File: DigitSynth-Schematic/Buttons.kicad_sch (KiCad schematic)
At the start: 16 parts

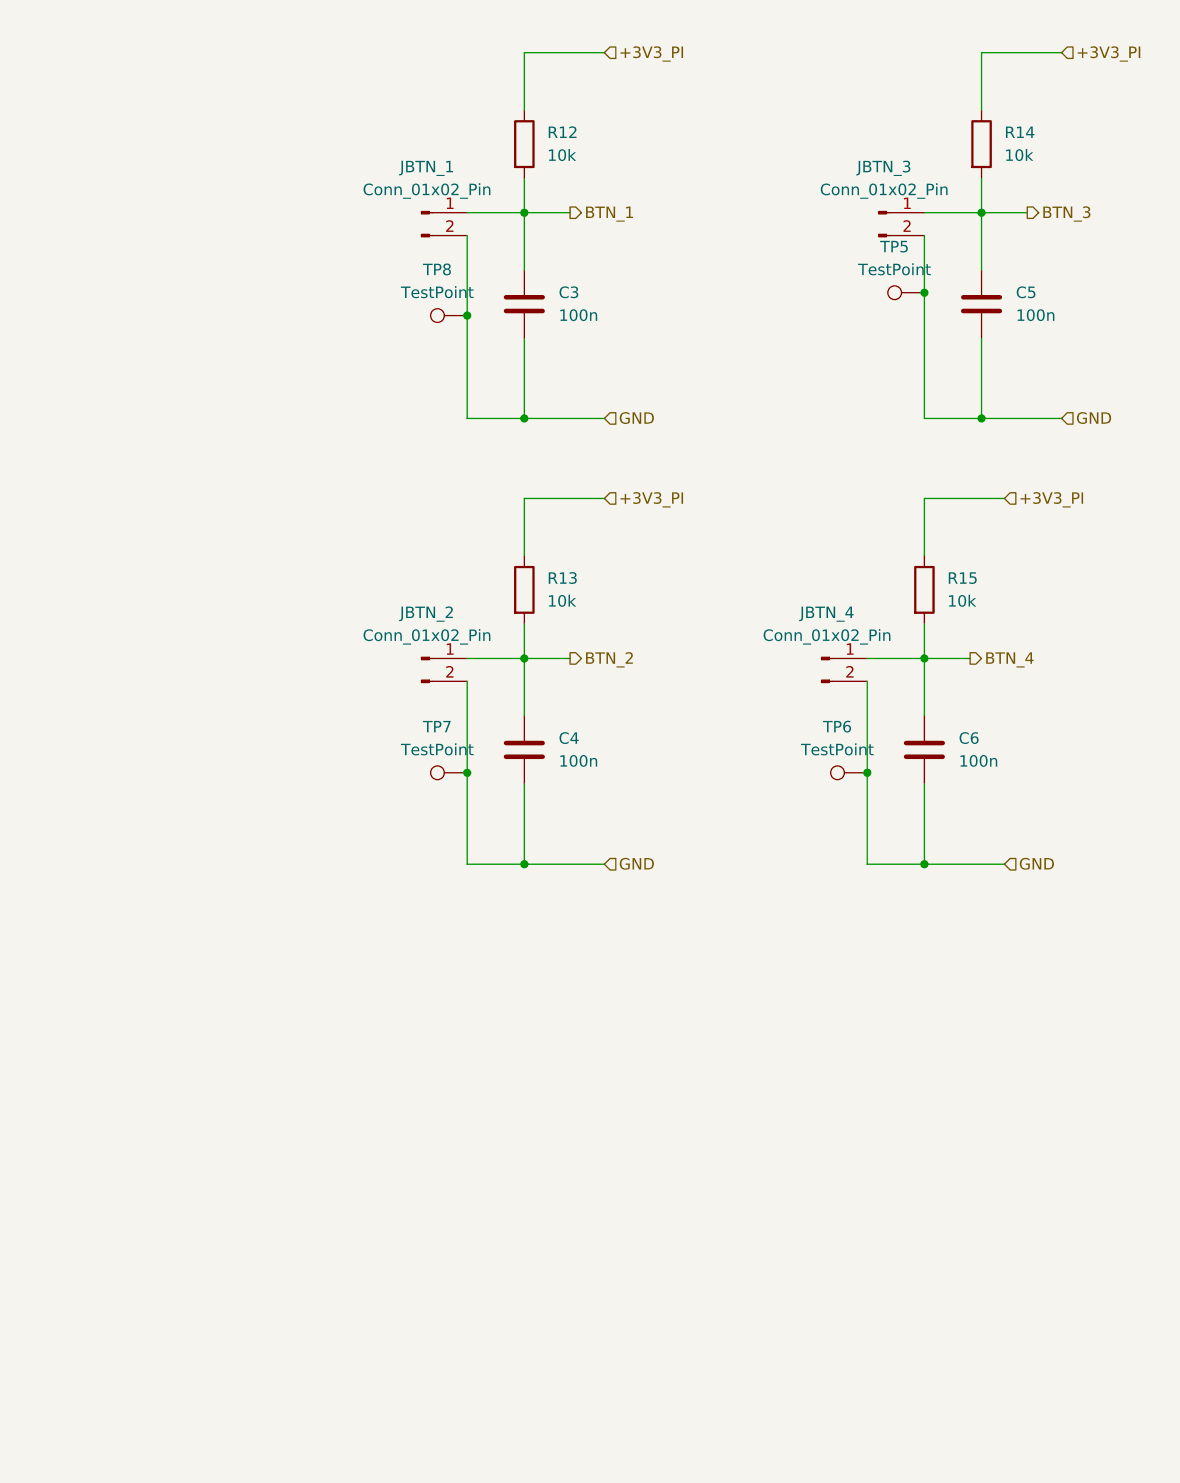
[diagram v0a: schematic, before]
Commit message: KiCad PCB fully routed
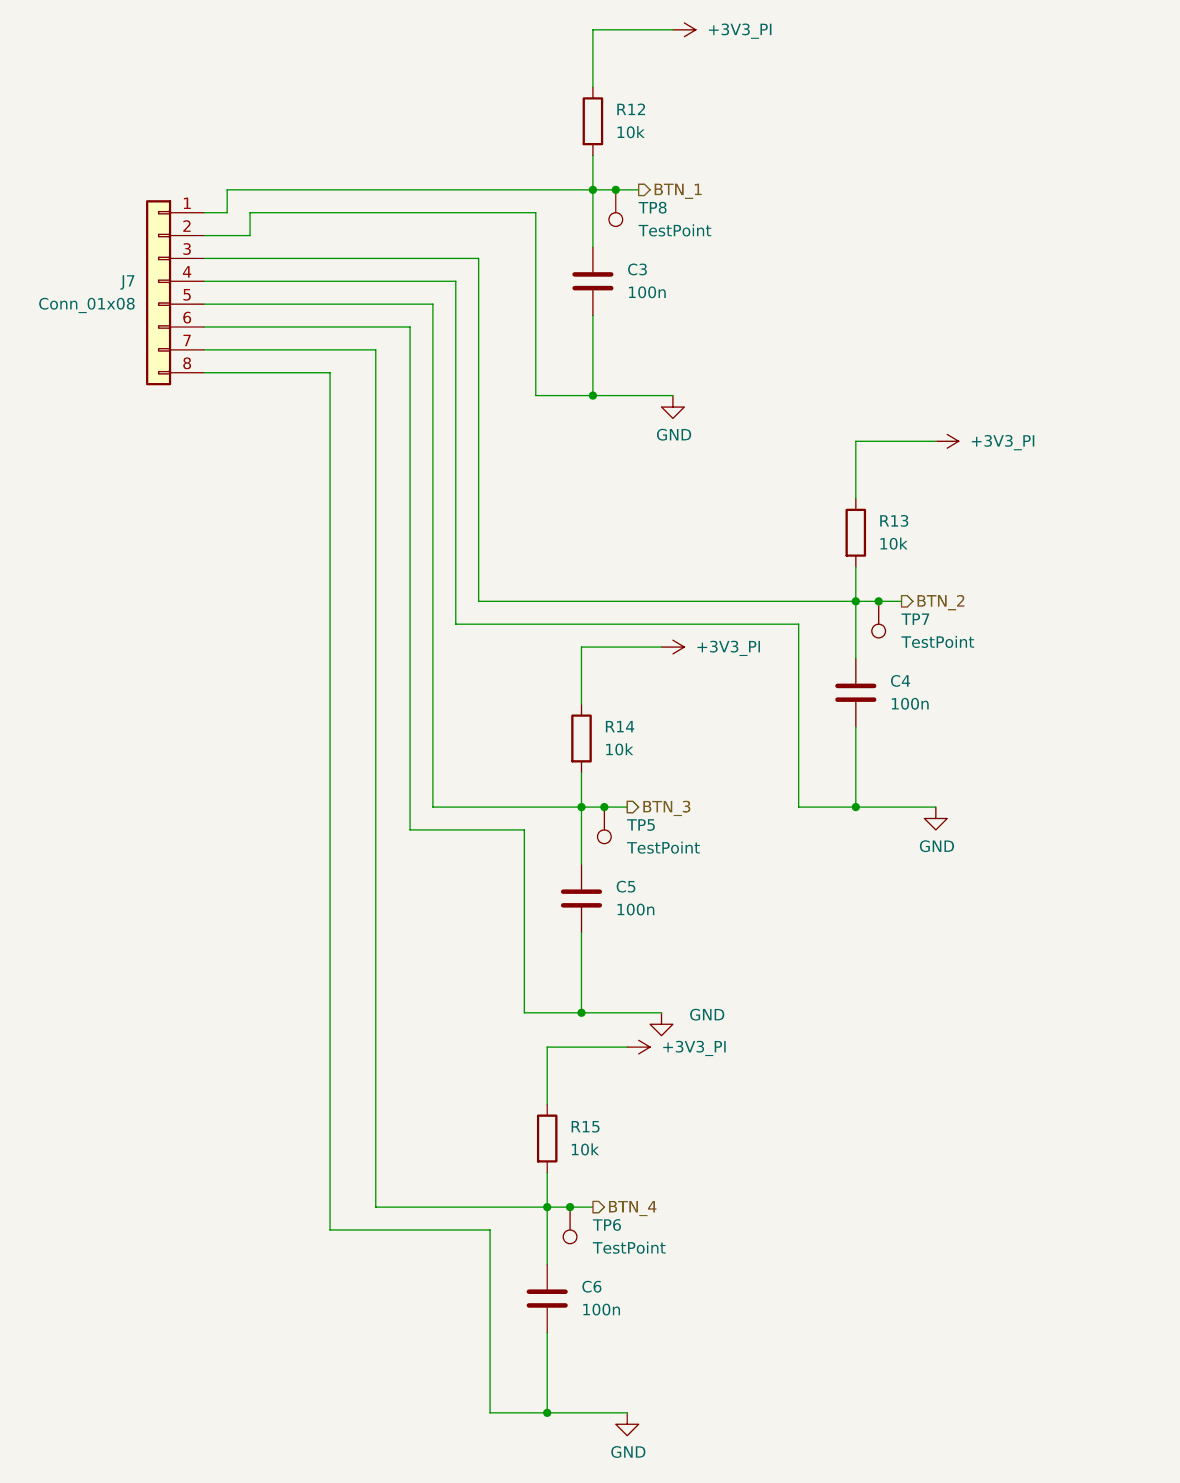
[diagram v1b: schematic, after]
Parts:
- removed JBTN_1, JBTN_2, JBTN_3, JBTN_4: Conn_01x02_Pin, symbol Connector:Conn_01x02_Pin
- added J7: Conn_01x08, Connector_Molex:Molex_KK-254_AE-6410-08A_1x08_P2.54mm_Vertical, symbol Connector_Generic:Conn_01x08
- C3, C4, C6: footprint (none) -> Capacitor_SMD:C_0603_1608Metric; LCSC Part # (none) -> C14663
- C5: footprint (none) -> Capacitor_SMD:C_0603_1608Metric; LSCS Part # (none) -> C14663
- R12, R13, R14, R15: footprint (none) -> Resistor_SMD:R_0603_1608Metric; LCSC Part # (none) -> C25804
- TP5, TP6, TP7, TP8: footprint (none) -> TestPoint:TestPoint_THTPad_D1.0mm_Drill0.5mm
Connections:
- net BTN_1: now also TP8.1, J7.1 (Pin_1)
- net BTN_2: now also TP7.1, J7.3 (Pin_3)
- net BTN_3: now also TP5.1, J7.5 (Pin_5)
- net BTN_4: now also TP6.1, J7.7 (Pin_7)
- net GND: now also J7.2 (Pin_2), J7.4 (Pin_4), J7.6 (Pin_6), J7.8 (Pin_8); no longer TP5.1, TP6.1, TP7.1, TP8.1
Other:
- moved on the sheet: C3, C4, C5, C6, R12, R13, R14, R15, TP5, TP6, TP7, TP8
